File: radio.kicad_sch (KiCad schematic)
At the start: 41 parts, among them J301 434MHz ANT pads, U301 CC1200, X301 40MHz

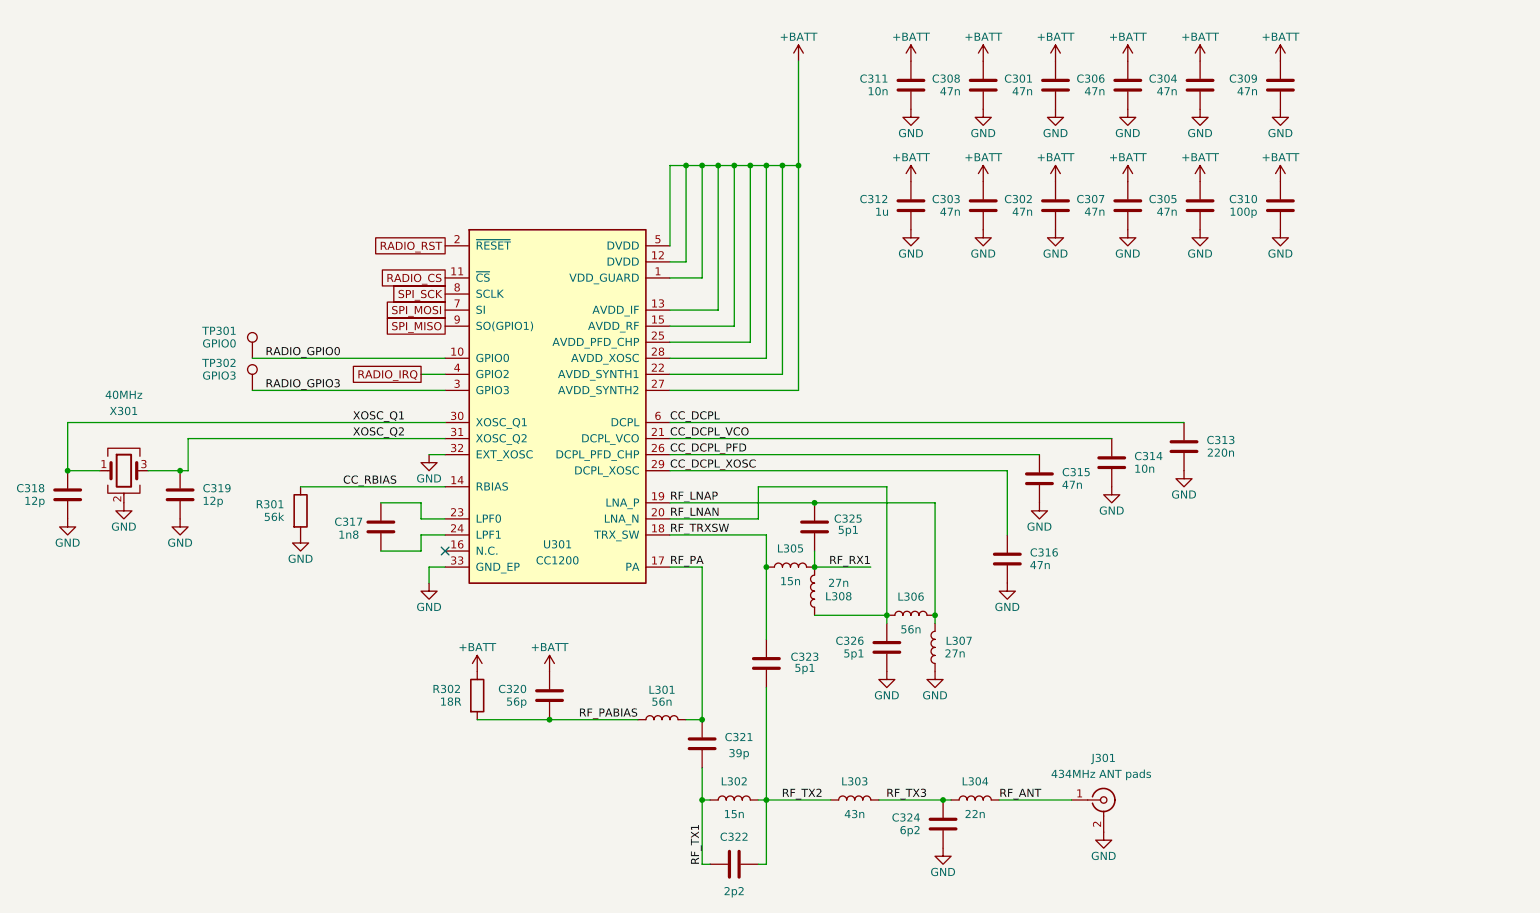
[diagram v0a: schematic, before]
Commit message: Inital routing
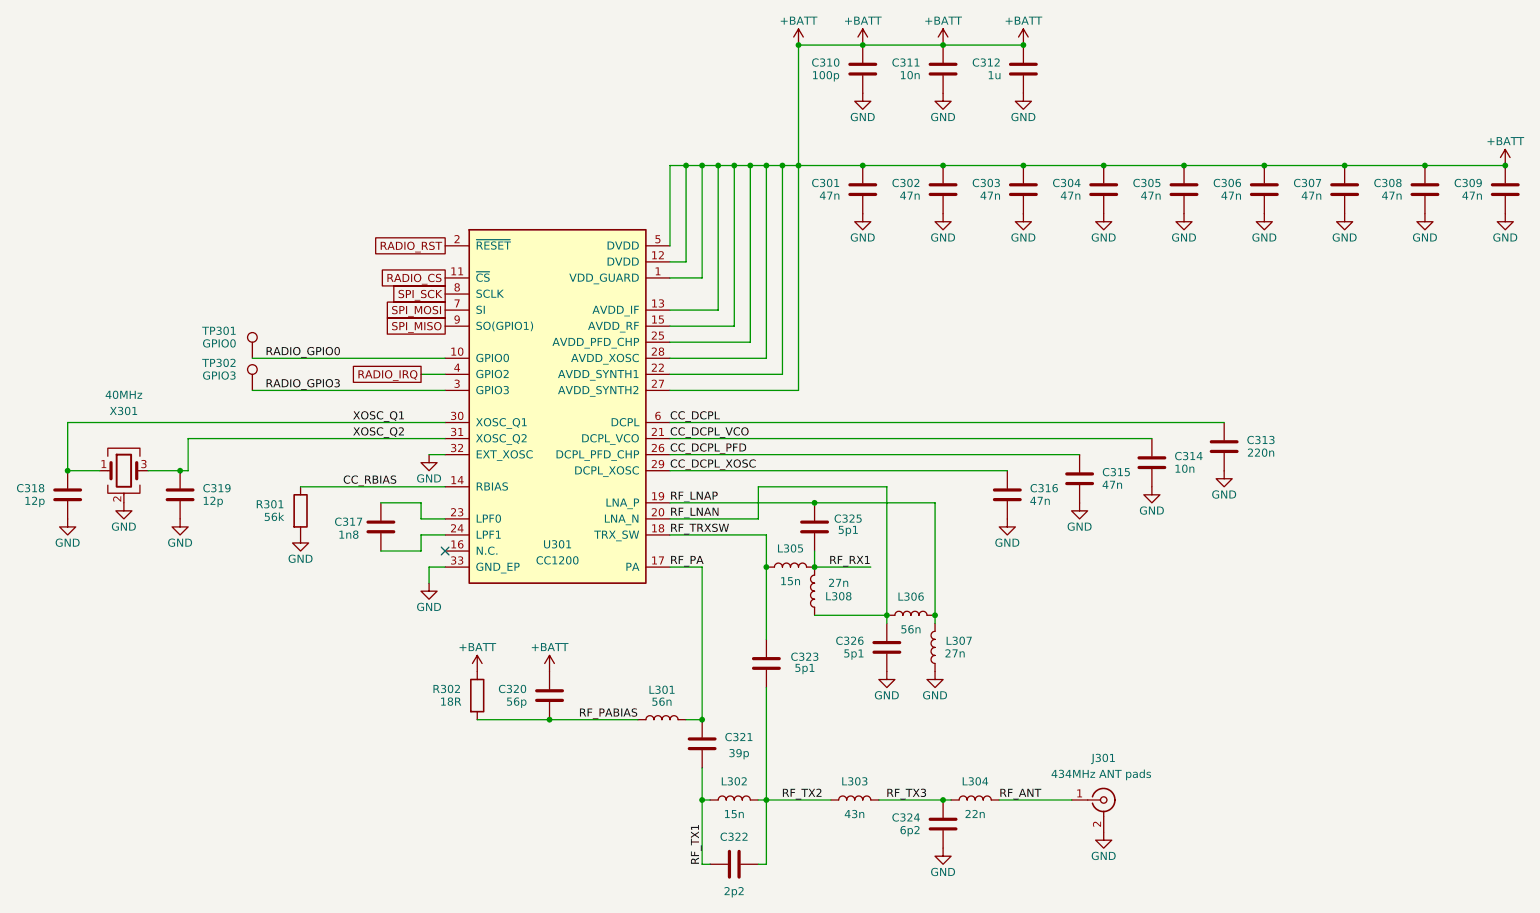
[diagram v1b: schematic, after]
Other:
- moved on the sheet: C301, C302, C303, C304, C305, C306, C307, C308, C309, C310, C311, C312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
